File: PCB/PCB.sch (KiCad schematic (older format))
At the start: 32 parts, among them J1 USB_B, U1 ESP32-WROOM-32, X1 12MHz

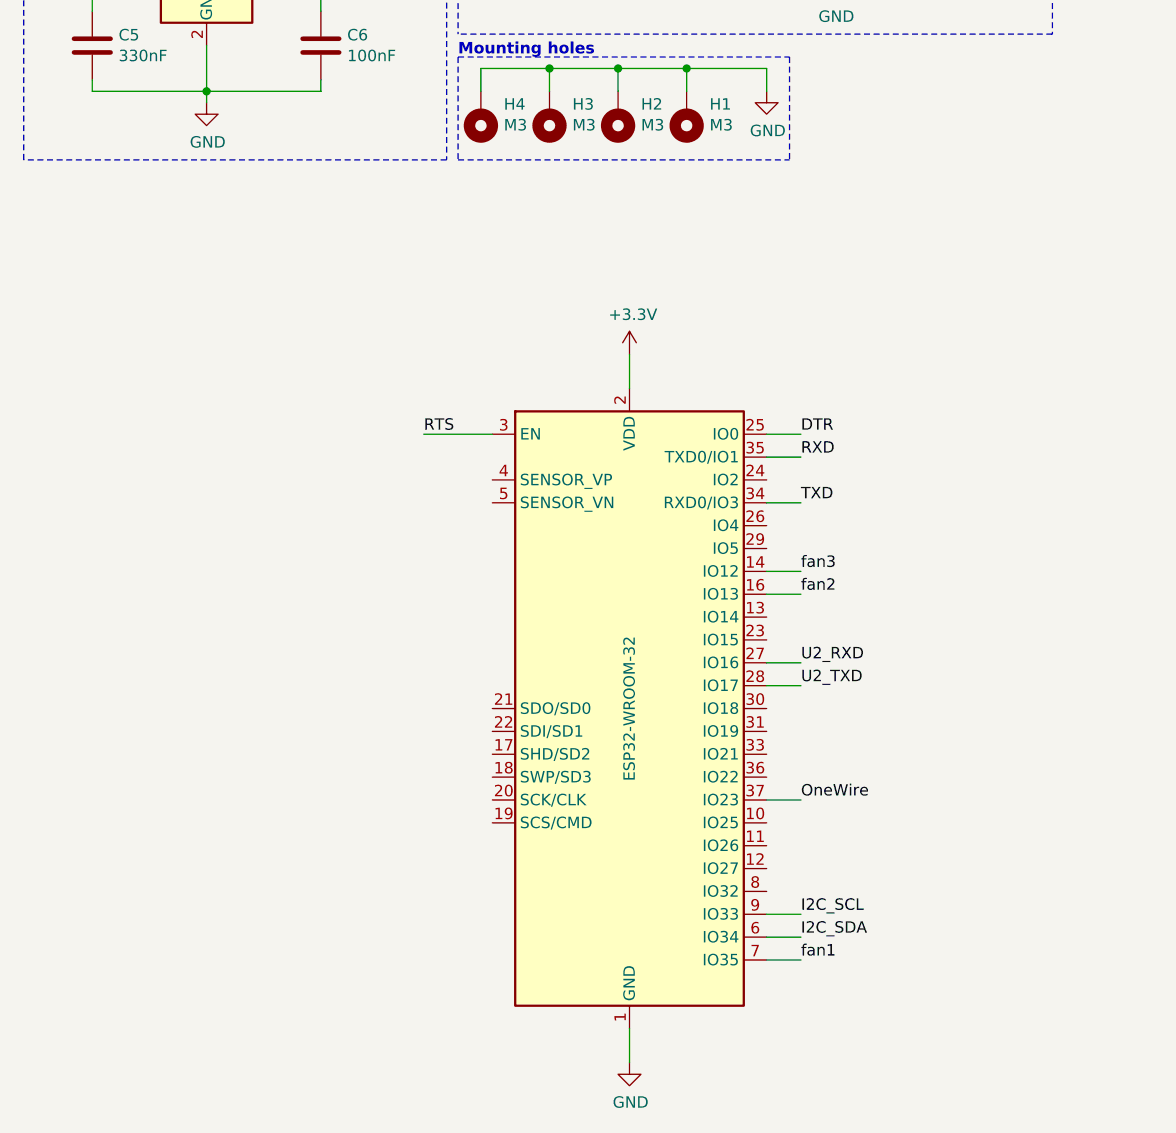
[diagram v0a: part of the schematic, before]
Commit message: LED indicator #4
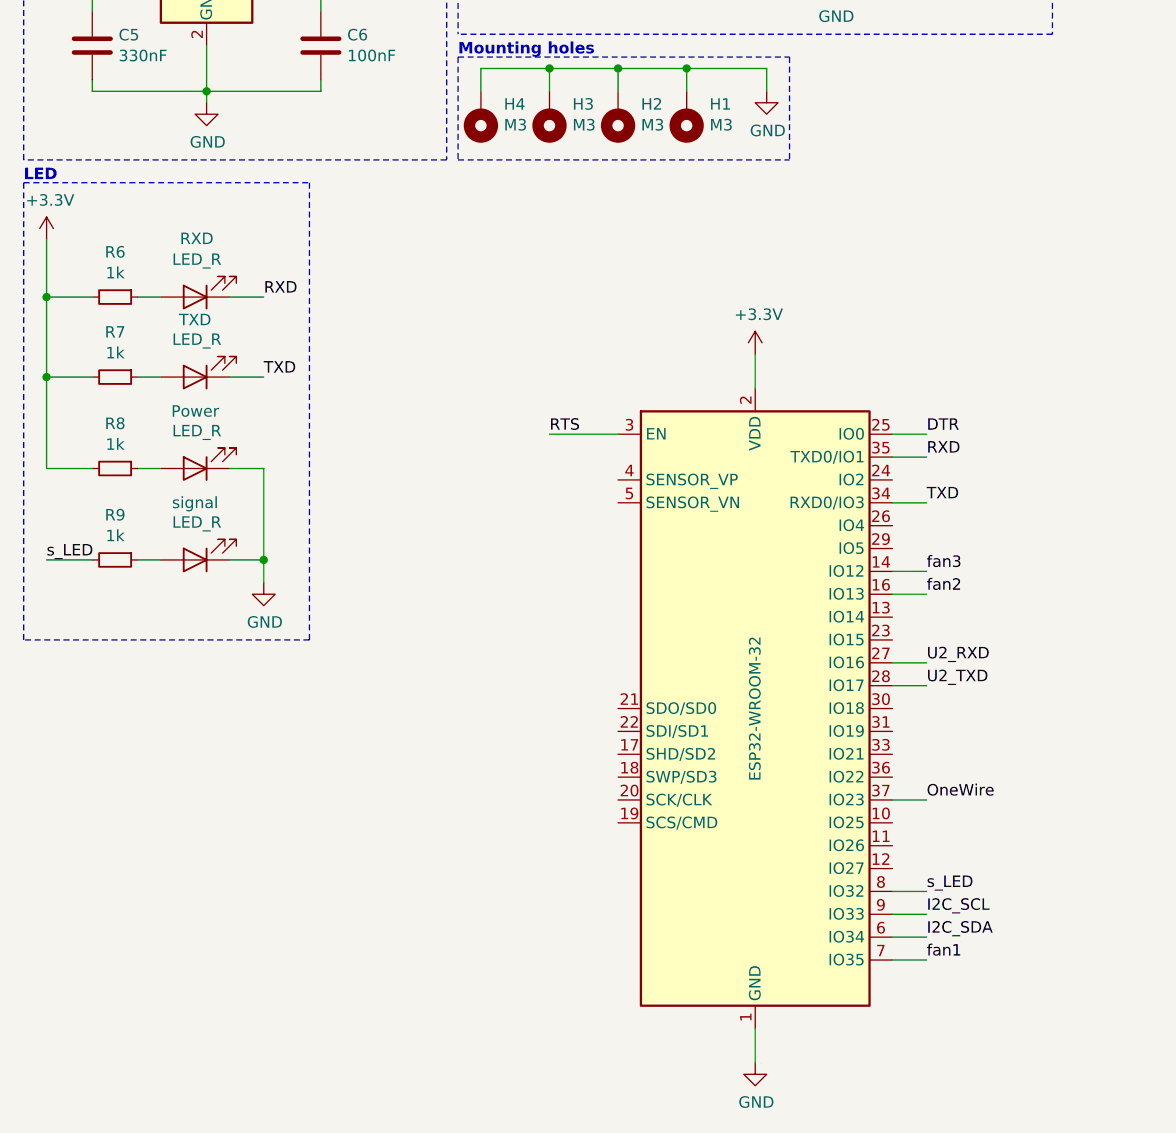
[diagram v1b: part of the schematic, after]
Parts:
- added Power, RXD, TXD, signal: LED_R, symbol Device:LED
- added R6, R7, R8, R9: 1k, Mlab_R:SMD-1206, symbol Device:R_Small
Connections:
- net +3V3: now also R6.2, R7.2, R8.2
- net GND: now also Power.1 (K), signal.1 (K)
- net RXD: now also RXD.1 (K)
- net TXD: now also TXD.1 (K)
- net s_LED: now reaches U1.8 (IO32)
- net s_LED: now also R9.2
- new net: R6.1, RXD.2 (A)
- new net: R7.1, TXD.2 (A)
- new net: Power.2 (A), R8.1
- new net: R9.1, signal.2 (A)
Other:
- note added: "LED"
